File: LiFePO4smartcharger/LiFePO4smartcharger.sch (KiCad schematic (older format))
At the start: 99 parts, among them J1 Conn_01x02, J10 Conn_01x01, J11 Conn_01x01, J12 Conn_01x04, J13 Conn_01x01, J2 Conn_02x03_Odd_Even, J3 Conn_01x02, J4 Conn_01x02, J5 Barrel_Jack, J6 Conn_01x01, J7 Conn_01x01, J8 Conn_01x02, J9 Conn_01x02, Q1 TIP42, Q2 TIP41, Q3 2N3906, Q4 TIP41C, T1 Transformer_1P1Sdotted, U1 ATMEGA328P-PU, U2 LM358, U3 LCD-016N002L, U4 TL494, U9 LM7805_TO220, X3 16MHz

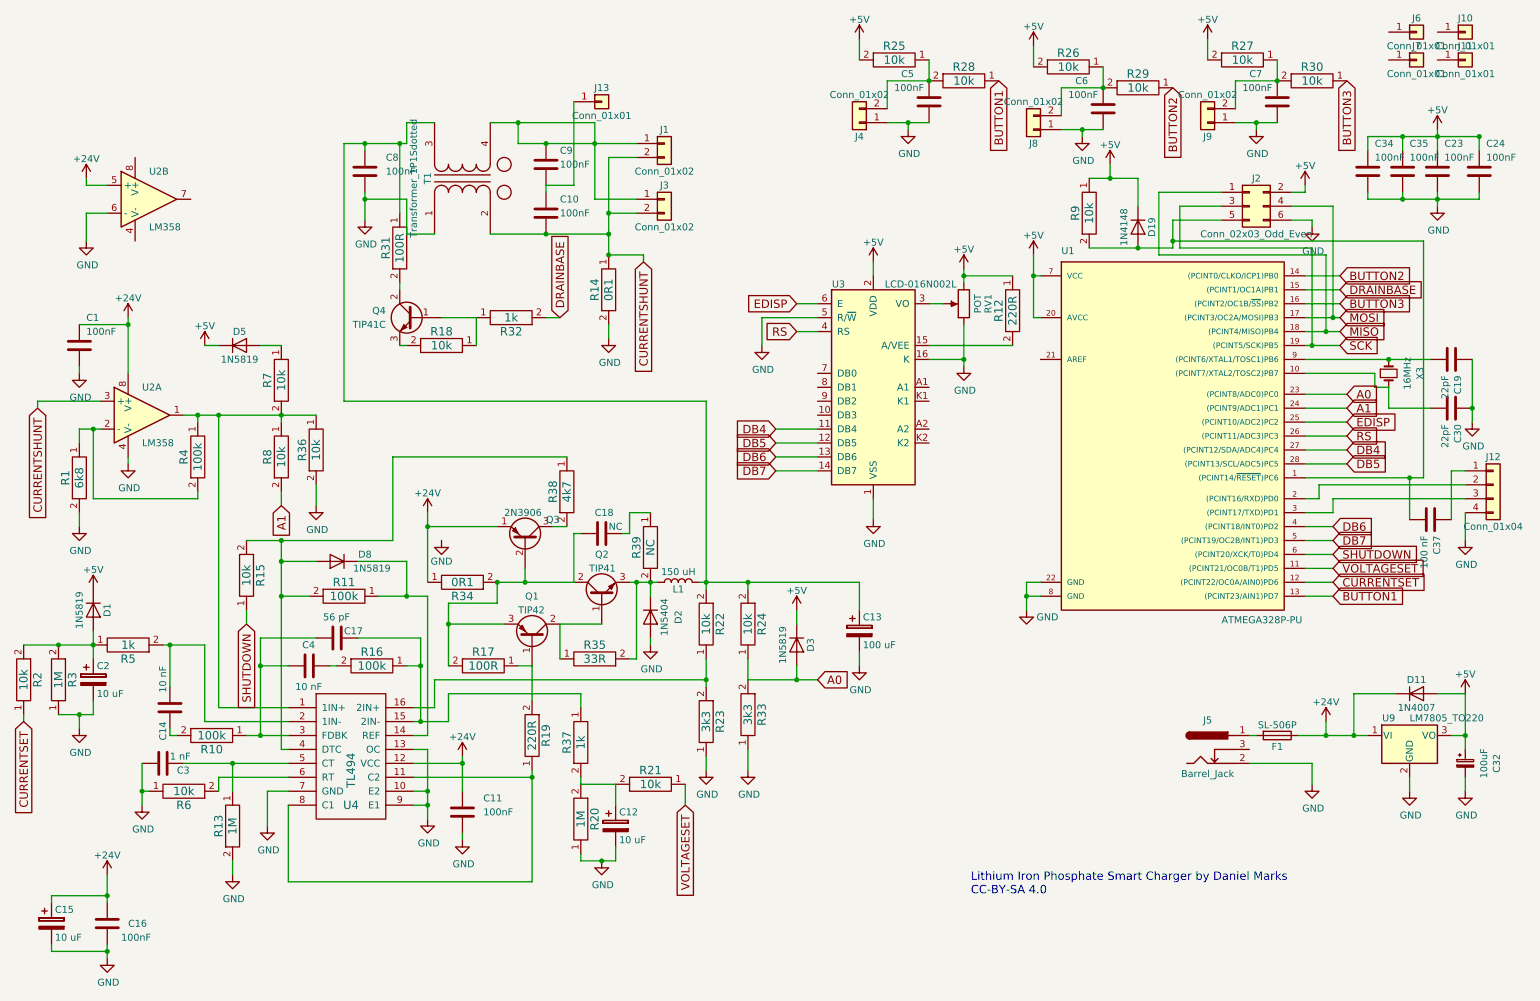
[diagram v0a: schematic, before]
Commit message: A few tweaks
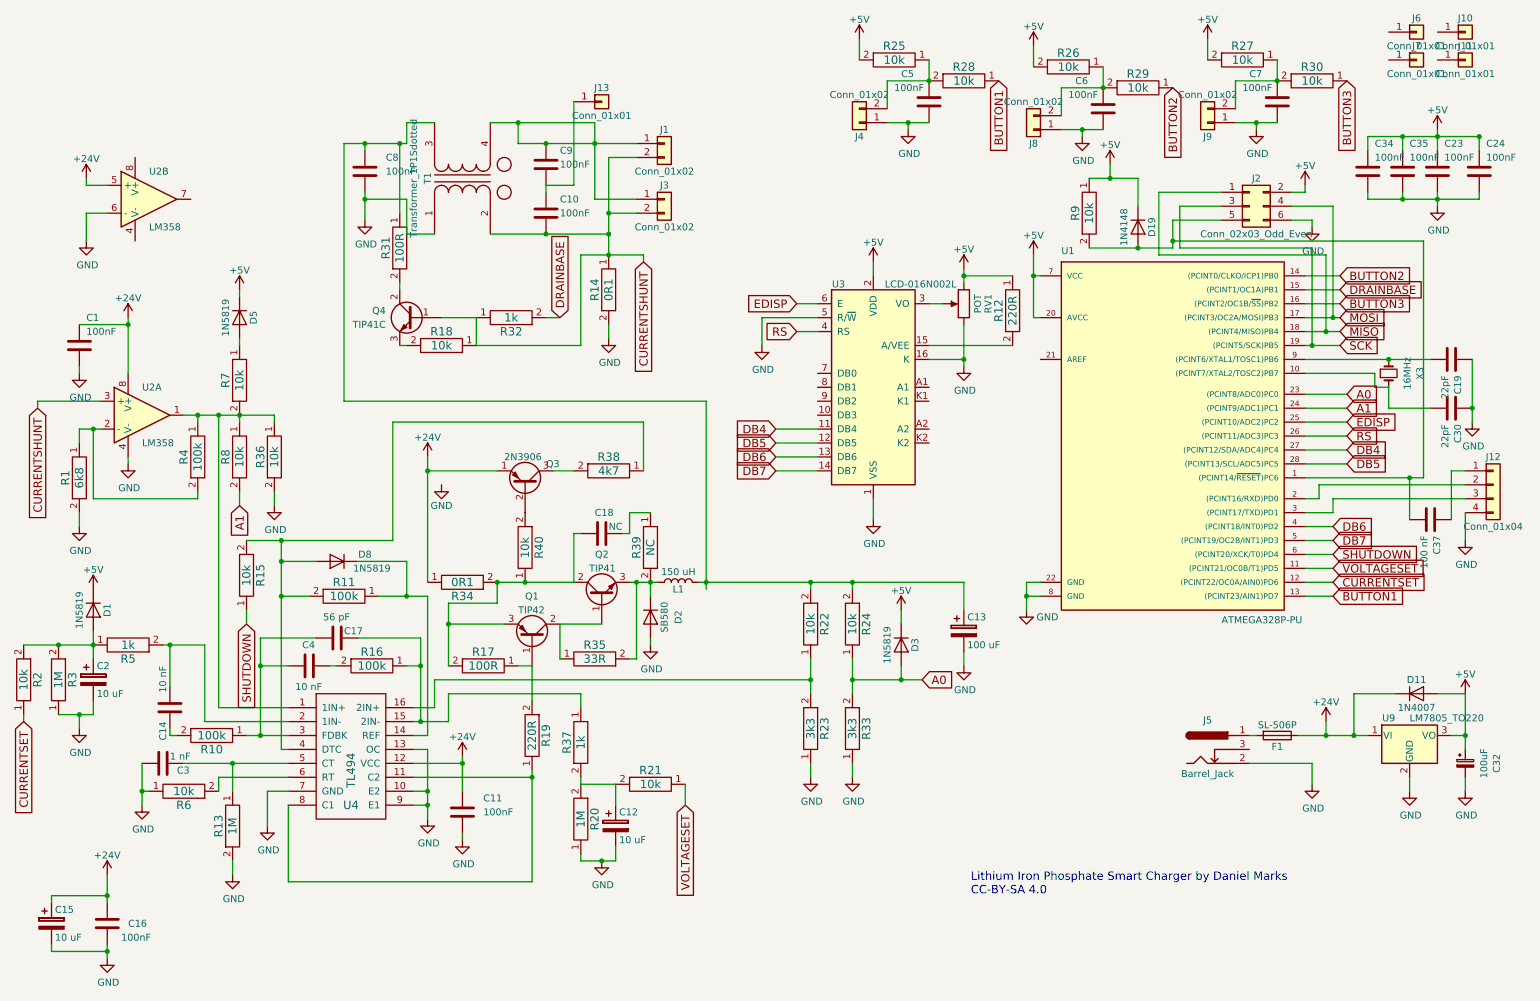
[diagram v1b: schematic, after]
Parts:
- added R40: 10k, Resistors_THT:R_Axial_DIN0207_L6.3mm_D2.5mm_P7.62mm_Horizontal, symbol RES
- D2: value 1N5404 -> SB580
- R19: footprint Resistors_THT:R_Axial_DIN0207_L6.3mm_D2.5mm_P7.62mm_Horizontal -> Resistors_THT:R_Axial_DIN0309_L9.0mm_D3.2mm_P12.70mm_Horizontal
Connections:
- net CURRENTSHUNT: now also Q4.1 (B), R18.1, R32.1
- net at C18.2, Q1.3 (E), Q2.2 (C)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: now also R40.1; no longer Q3.2 (B)
- new net: Q3.2 (B), R40.2
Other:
- moved on the sheet: C13, D3, D5, Q3, R22, R23, R24, R33, R38, R7, R8
